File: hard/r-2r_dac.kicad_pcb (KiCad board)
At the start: 2 copper layers, 109.2 x 58.4 mm, 45 parts, among them J1 Conn_01x04_Male, J2 Conn_01x08_Male, J3 Conn_01x01_Male, J4 Conn_01x01_Male, J5 Conn_01x01_Male, J6 Conn_01x02_Male, Q1 BD135, Q2 BD136, U1 L78L33_TO92, U2 74HC595, U3 LM358

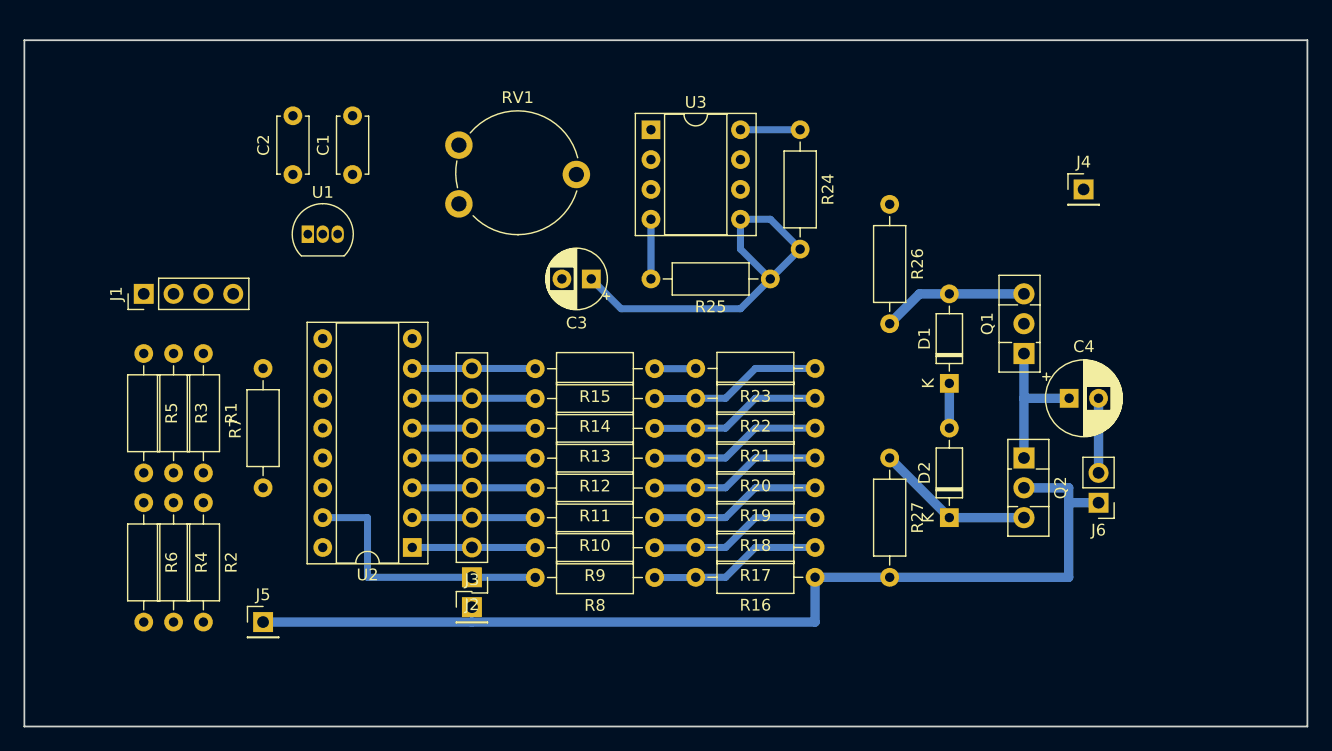
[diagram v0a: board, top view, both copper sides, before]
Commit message: in work
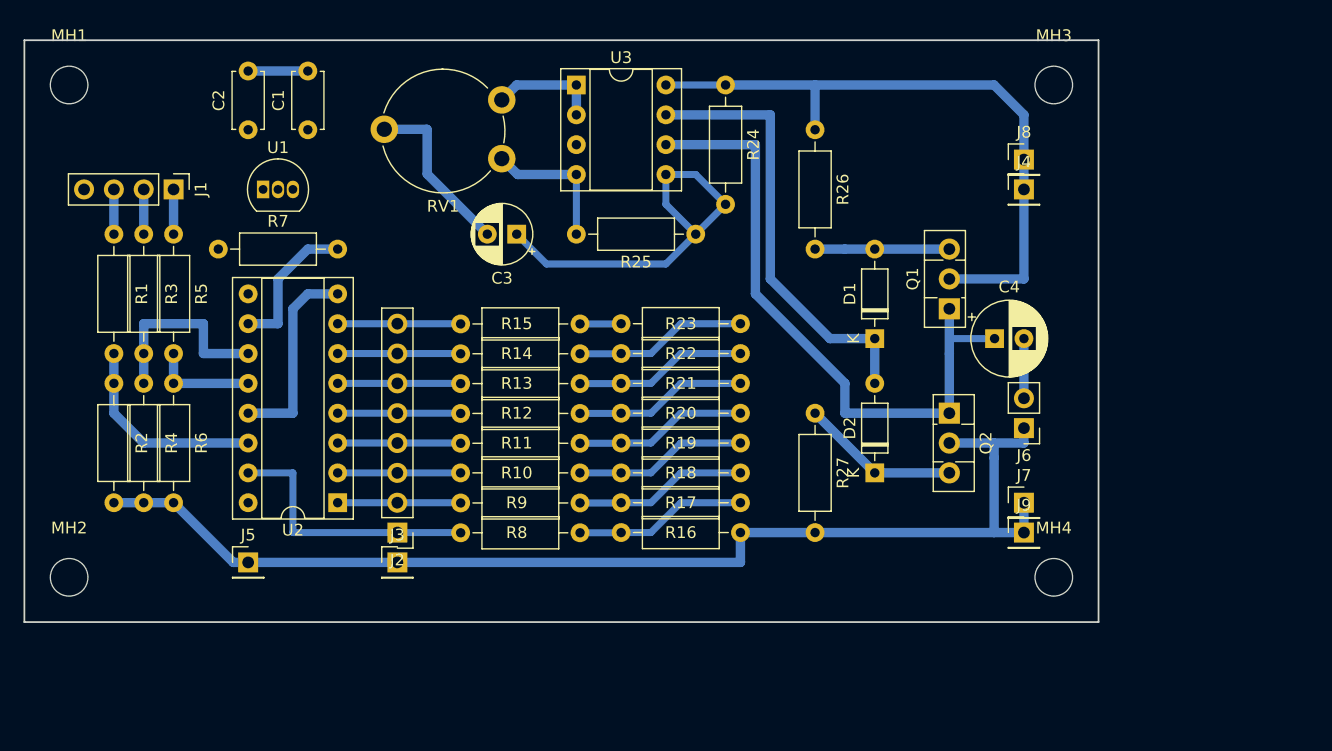
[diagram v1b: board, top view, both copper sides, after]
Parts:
- added J7: Conn_01x01_Male, Connector_PinHeader_2.54mm:PinHeader_1x01_P2.54mm_Vertical, F.Cu at (138.4, 86.4)
- added J8: Conn_01x01_Male, Connector_PinHeader_2.54mm:PinHeader_1x01_P2.54mm_Vertical, F.Cu at (138.4, 57.1)
- added J9: Conn_01x01_Male, Connector_PinHeader_2.54mm:PinHeader_1x01_P2.54mm_Vertical, F.Cu at (138.4, 88.9)
- added MH1: MountingHole, MountingHole:MountingHole_3.2mm_M3, F.Cu at (57.1, 50.8)
- added MH2: MountingHole, MountingHole:MountingHole_3.2mm_M3, F.Cu at (57.1, 92.7)
- added MH3: MountingHole, MountingHole:MountingHole_3.2mm_M3, F.Cu at (141.0, 50.8)
- added MH4: MountingHole, MountingHole:MountingHole_3.2mm_M3, F.Cu at (141.0, 92.7)
- moved R7 20.7 mm to (69.8, 64.8), turned to 0 degrees
- moved R1 12.7 mm to (61.0, 63.5)
- moved R2 12.7 mm to (61.0, 76.2)
- moved R3 10.5 mm to (63.5, 63.5)
- moved R4 10.5 mm to (63.5, 76.2)
- moved R5 10.5 mm to (66.0, 63.5)
- moved R6 10.5 mm to (66.0, 76.2)
- moved RV1 9.57 mm to (94.0, 52.1), turned to 180 degrees
- moved J1 9.25 mm to (66.0, 59.7), turned to 270 degrees
- moved R26 8.98 mm to (120.7, 54.6)
- moved J6 8.98 mm to (138.4, 80.0)
- moved C4 8.13 mm to (135.9, 72.4)
- moved D1 7.41 mm to (125.7, 72.4)
- moved D2 7.41 mm to (125.7, 83.8)
- moved R10 7.41 mm to (100.6, 83.8)
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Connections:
- RV1 pad 1: GND -> Net-(RV1-Pad1)
- RV1 pad 3: Net-(RV1-Pad3) -> GND
- U3 pad 1: Net-(RV1-Pad3) -> Net-(RV1-Pad1)
- U3 pad 2: Net-(RV1-Pad3) -> Net-(RV1-Pad1)
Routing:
- net VCC: track 5.08 -> 55.7 mm
- net GND: track 91.4 -> 134.0 mm
- net Net-(C4-Pad1): track 12.7 -> 55.3 mm
- net Net-(D1-Pad1): track 3.81 -> 37.7 mm
- net Net-(R1-Pad2): track 0.00 -> 17.6 mm
- net Net-(R3-Pad2): track 0.00 -> 16.5 mm
- net Net-(C3-Pad2): track 0.00 -> 14.7 mm
- net Net-(R7-Pad2): track 0.00 -> 12.5 mm
- net Net-(RV1-Pad1): track 0.00 -> 9.42 mm
- net Net-(R5-Pad2): track 0.00 -> 8.89 mm
- net Net-(J1-Pad3): track 0.00 -> 3.81 mm
- net Net-(J1-Pad2): track 0.00 -> 3.81 mm
- net Net-(J1-Pad1): track 0.00 -> 3.81 mm
- net Net-(C4-Pad2): track 6.35 -> 5.08 mm
- net Net-(D1-Pad2): track 12.5 -> 11.4 mm
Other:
- board size 109.2 x 58.4 mm -> 91.4 x 49.5 mm
